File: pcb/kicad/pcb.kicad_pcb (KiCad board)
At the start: 2 copper layers, 56.3 x 62.8 mm, 45 parts, among them J1 Raspberry_Pi_2_3, U1 MCP4822, U2 TL082, U3 TL082, U4 LM358, U5 ADC0831, U6 AOZ1282CI

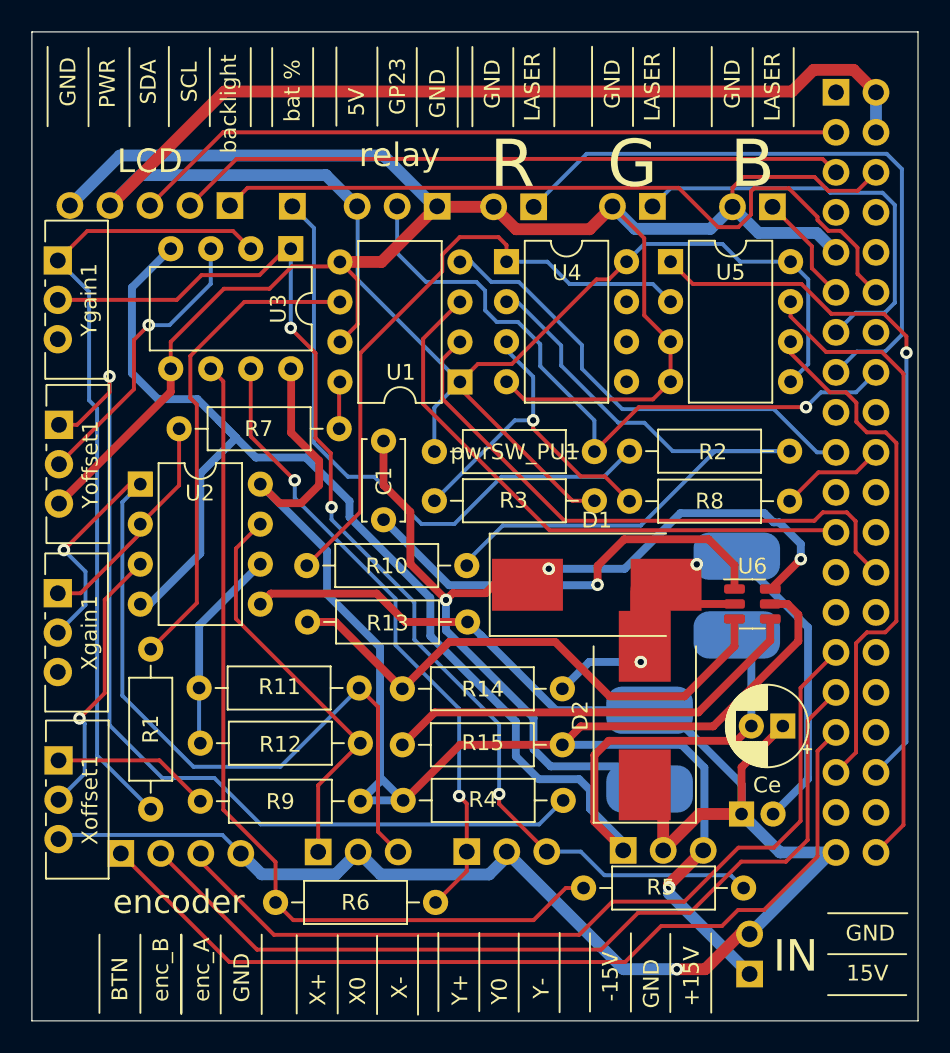
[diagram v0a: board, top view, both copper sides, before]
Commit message: smd pcb done
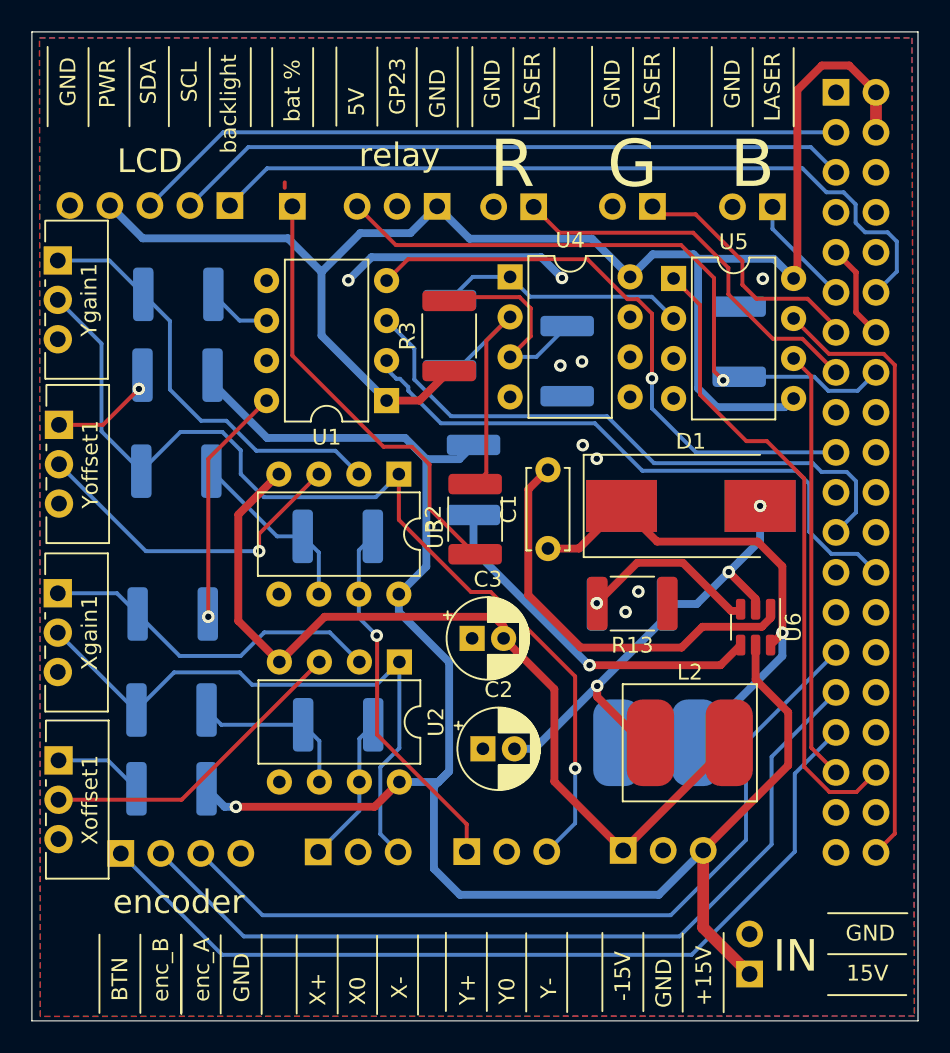
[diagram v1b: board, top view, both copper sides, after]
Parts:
- removed Ce: 10u, Capacitor_THT:CP_Radial_D5.0mm_P2.00mm
- added C3: 10u, Capacitor_THT:CP_Radial_D5.0mm_P2.00mm, F.Cu at (253.8, 60.1)
- C2, L2: moved to F.Cu
- D2: moved to B.Cu
- R1, R10, R11, R12, R14, R15, R4, R5, R6, R7, R8, R9, pwrSW_PU1: footprint Resistor_THT:R_Axial_DIN0207_L6.3mm_D2.5mm_P10.16mm_Horizontal -> Resistor_SMD:R_1812_4532Metric_Pad1.30x3.40mm_HandSolder; moved to B.Cu
- R13, R2, R3: footprint Resistor_THT:R_Axial_DIN0207_L6.3mm_D2.5mm_P10.16mm_Horizontal -> Resistor_SMD:R_1812_4532Metric_Pad1.30x3.40mm_HandSolder
- moved R5 37.0 mm to (235.0, 49.5), turned to 180 degrees
- moved R1 32.7 mm to (235.1, 38.2), turned to 0 degrees
- moved R4 30.6 mm to (235.1, 43.4), turned to 180 degrees
- moved R6 24.1 mm to (245.2, 53.6)
- moved pwrSW_PU1 20.6 mm to (270.7, 41.2), turned to -90 degrees
- moved U2 20.0 mm to (249.1, 61.6), turned to -90 degrees
- moved R15 17.4 mm to (253.8, 50.0), turned to 90 degrees
- moved C2 16.9 mm to (254.4, 67.1)
- moved R8 16.7 mm to (259.8, 42.5), turned to 90 degrees
- moved U3 15.9 mm to (249.1, 49.6)
- moved R14 15.5 mm to (263.9, 57.9)
- moved R10 14.7 mm to (252.3, 40.8), turned to 90 degrees
- moved R3 13.9 mm to (252.3, 40.9), turned to 90 degrees
- moved D2 13.6 mm to (267.6, 51.7), turned to 0 degrees
- moved C1 12.5 mm to (258.6, 54.4), turned to 90 degrees
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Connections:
- pwrSW1 pad 1: GND -> +5V
- pwrSW1 pad 2: Net-(J1-Pad16) -> GND
- pwrSW1 pad 3: +5V -> Net-(J1-Pad16)
- pwrSW_PU1 pad 1: +5V -> GND
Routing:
- net GND: track 257.6 -> 20.8 mm, vias 1 -> 9
- net Net-(R4-Pad2): track 59.3 -> 6.04 mm
- net Net-(R5-Pad1): track 56.5 -> 11.6 mm
- net -15V: track 95.7 -> 56.7 mm
- net +5V: track 137.1 -> 100.6 mm
- net Net-(R10-Pad1): track 46.3 -> 16.8 mm
- net Net-(R1-Pad2): track 30.9 -> 4.07 mm
- net Net-(C1-Pad1): track 59.5 -> 34.1 mm, vias 3 -> 1
- net Net-(R10-Pad2): track 40.6 -> 15.9 mm
- net Net-(R1-Pad1): track 50.8 -> 27.3 mm
- net Net-(R13-Pad2): track 34.6 -> 11.6 mm, vias 0 -> 1
- net Net-(R11-Pad2): track 57.4 -> 38.7 mm, vias 1 -> 0
- net Net-(R6-Pad1): track 41.1 -> 23.2 mm, vias 2 -> 1
- net Net-(J1-Pad15): track 40.9 -> 24.5 mm
- net Net-(R12-Pad1): track 25.8 -> 9.52 mm
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- added copper zone on B.Cu, net GND
- added copper zone on F.Cu, net GND
